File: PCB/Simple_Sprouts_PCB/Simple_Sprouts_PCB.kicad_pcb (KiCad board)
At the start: 4 copper layers, 69 x 70.6 mm, 43 parts, among them J1 Raspberry_Pi_5, J12 12V, J2 12V IN, J3 Soil Sensor, J4 Soil Sensor, J5 5V IN, J6 Temperature Sensor, J7 Air Quality Sensor, J8 Humidity Sensor, J9 HC-SR04, Q1 IRLB8721PbF, Q2 IRLB8721PbF, Q3 IRLB8721PbF, Q4 IRLB8721PbF, Q5 IRLB8721PbF, Q6 IRLB8721PbF

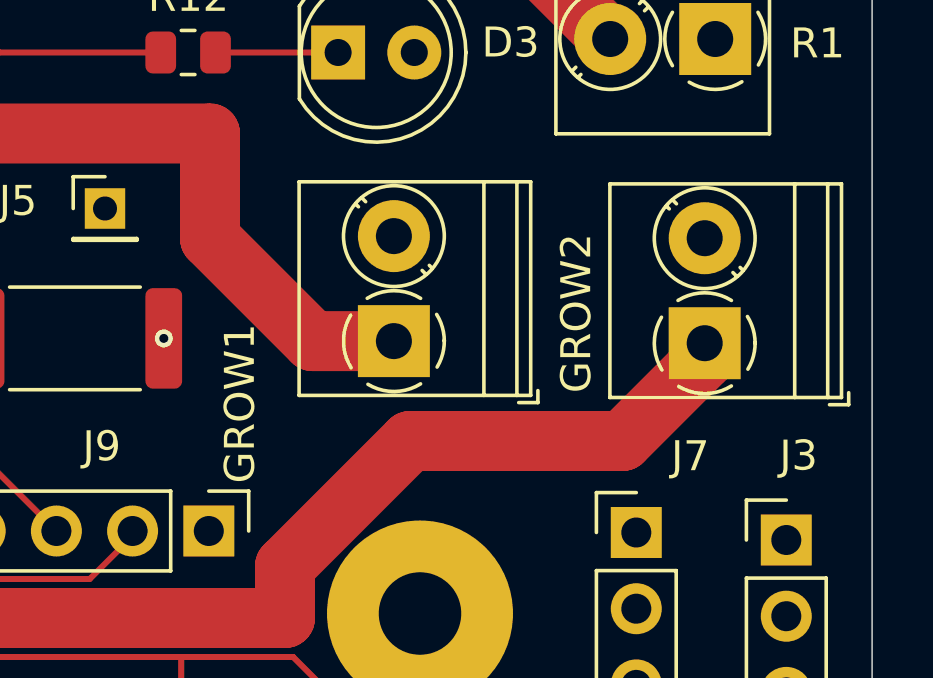
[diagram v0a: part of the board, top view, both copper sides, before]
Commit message: Add files via upload
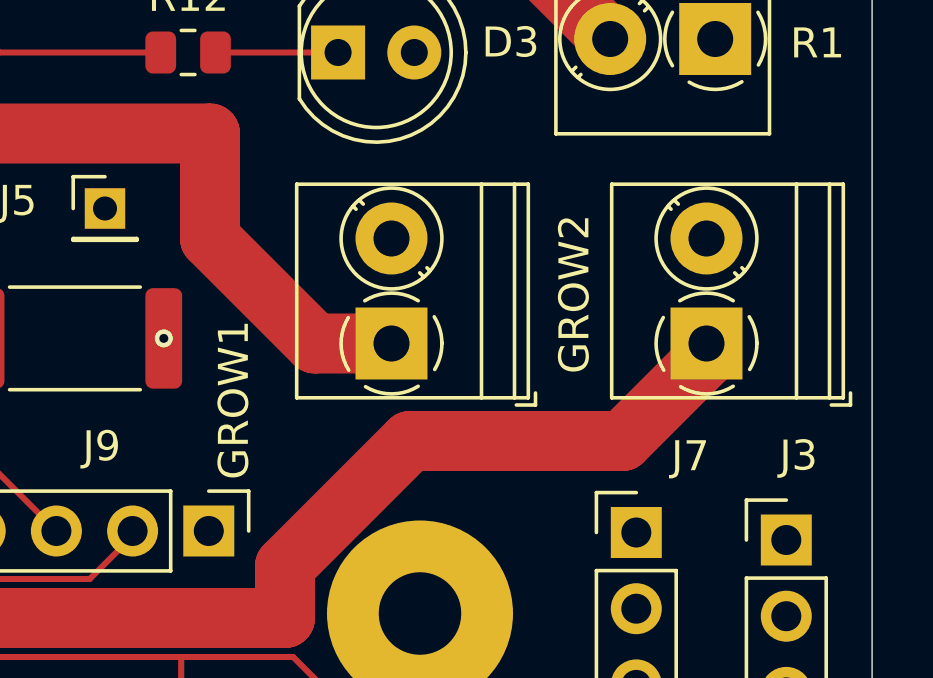
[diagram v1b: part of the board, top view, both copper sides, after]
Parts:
- moved GROW1 0.11 mm to (171.1, 114.0)
- moved GROW2 0.06 mm to (181.6, 114.0)
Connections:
- GROW1 pad 1: (no net) -> Net-(Q3-D)
- GROW1 pad 2: (no net) -> +5V
- GROW2 pad 1: (no net) -> Net-(Q2-D)
- GROW2 pad 2: (no net) -> +5V
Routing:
- net +5V: track 113.6 -> 110.9 mm
